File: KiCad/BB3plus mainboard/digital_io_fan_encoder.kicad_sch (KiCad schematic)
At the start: 50 parts, among them IC10 EMC2301-1-ACZL-TR, IC11 ISO6763FDWR, IC12 BD00FC0W, IC13 THVD1420DR, IC14 TPD4E001DRLR, IC15 TPD4E001DRLR, SW2 PEC16-2215F-S0024, X12 22-27-2031, X13 TBP03R1-350-10BE

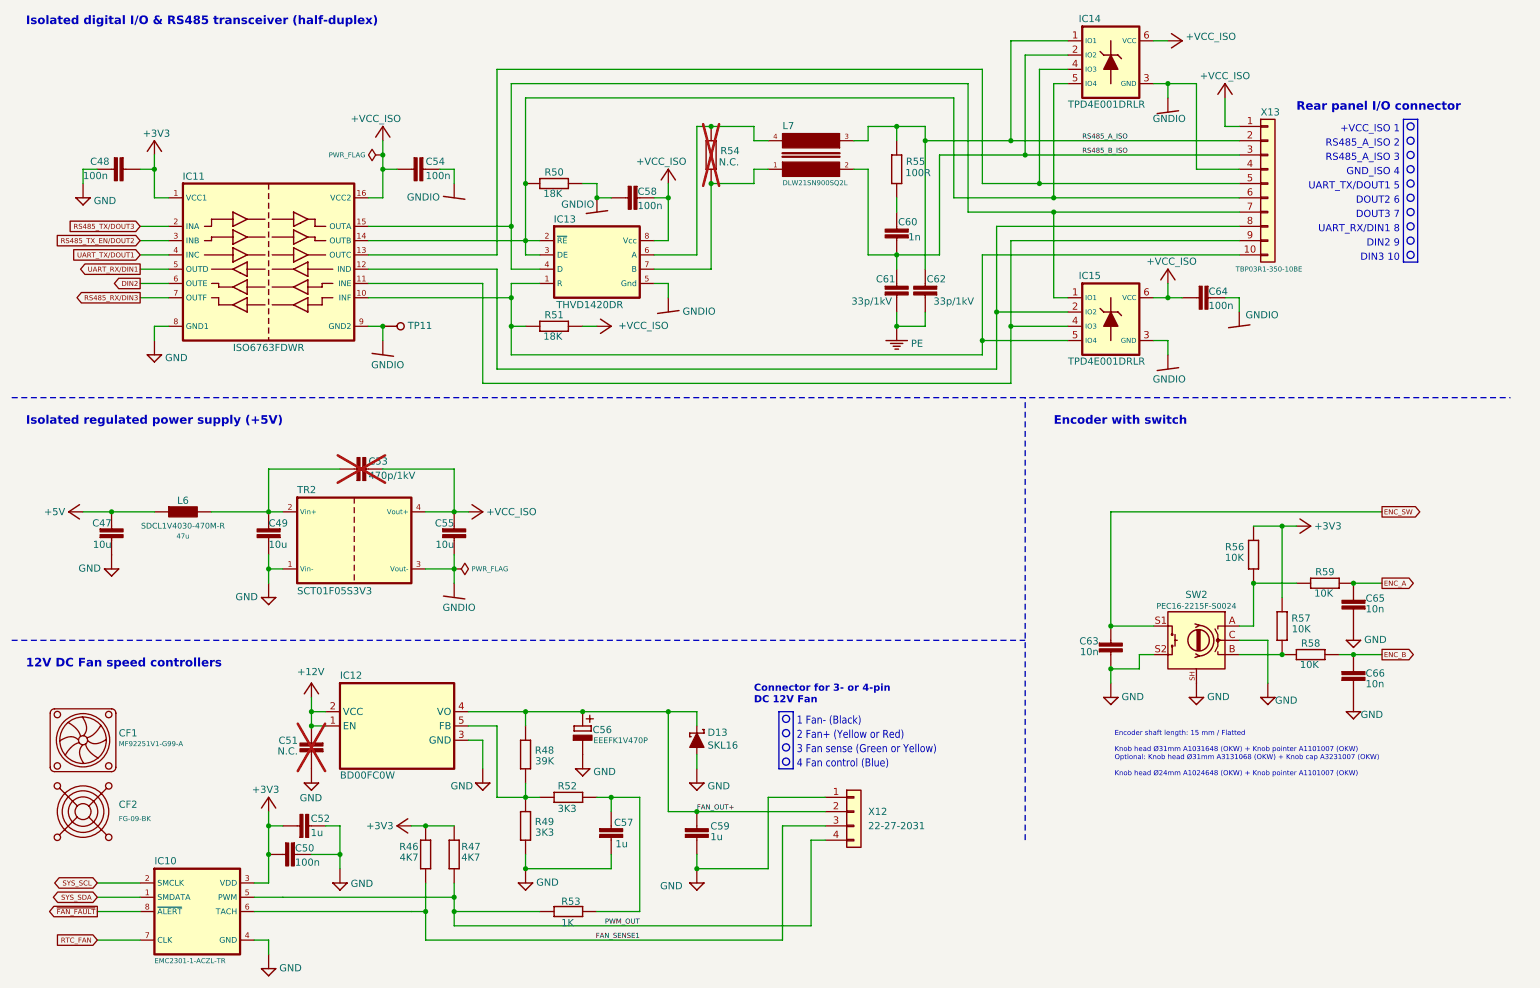
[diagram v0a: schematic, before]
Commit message: TOUT connected
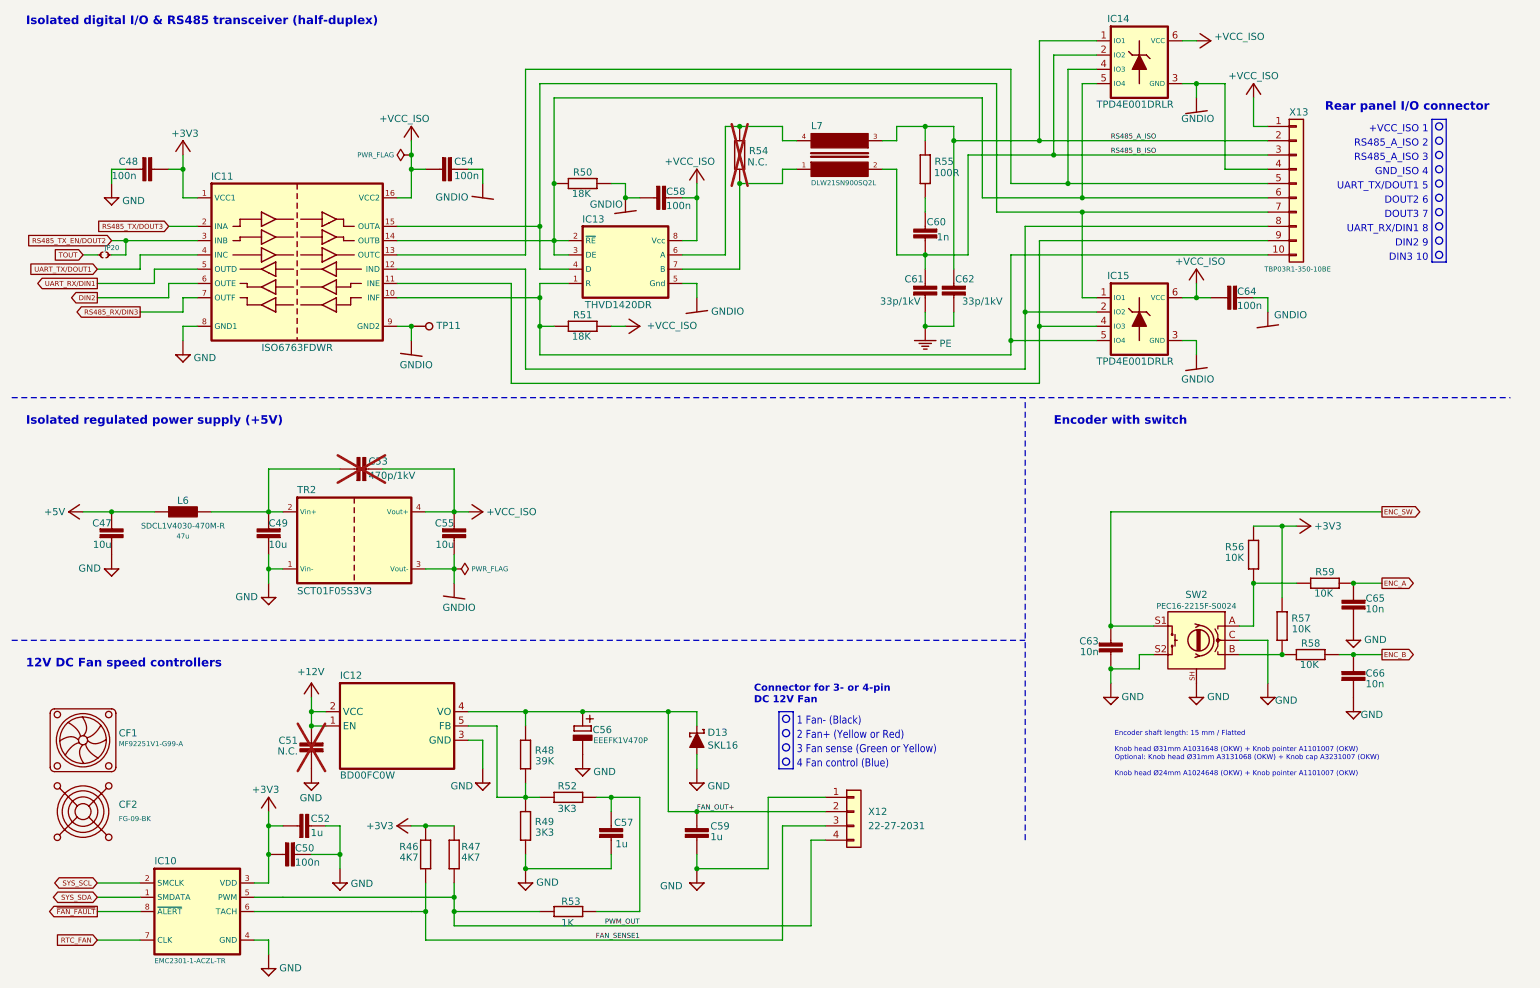
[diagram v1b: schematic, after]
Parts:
- added JP20: (no value), PCM_EEZ_SMD:JP2 open (0603), symbol PCM_EEZ_unsorted:JP2 open
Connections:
- net RS485_TX_EN/DOUT2: now also JP20.2
- new net TOUT: JP20.1
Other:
- moved on the sheet: C48, C54, C58, C60, C61, C62, C64, IC11, IC13, IC14, IC15, L7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
